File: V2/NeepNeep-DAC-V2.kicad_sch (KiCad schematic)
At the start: 18 parts, among them J1 Conn_02x03_Odd_Even, Q1 MMBT3904, U2 W25Q32JVSS, U3 ATtiny85-20SU

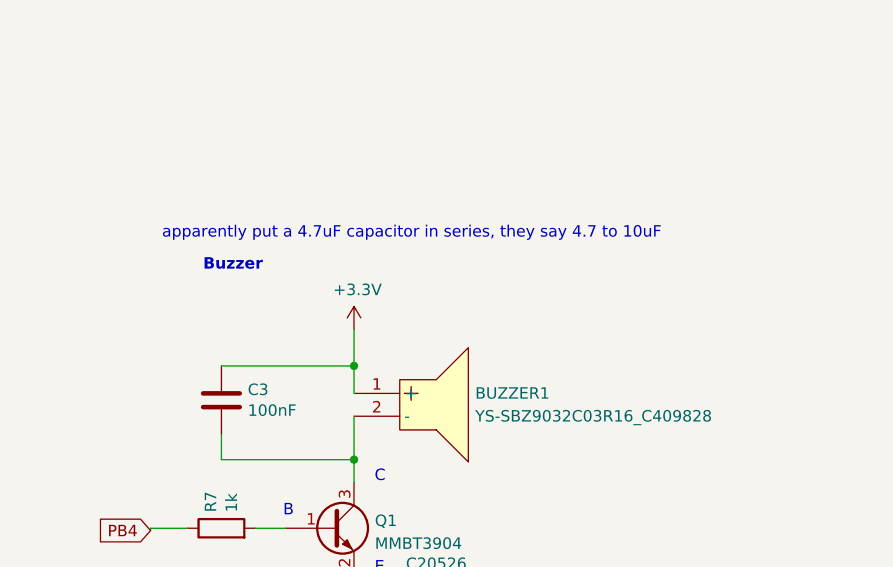
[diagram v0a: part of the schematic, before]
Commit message: Commit: M	NeepNeep-DAC-V1.kicad_sch A	V2/NeepNeep-DAC-V2-backups/NeepNeep-DAC-V2-2026-02-05_161125.zip A	V2/NeepNeep-DAC-V2-backups/NeepNeep-DAC-V2-2026-02-05_170153.zip A	V2/NeepNeep-DAC-V2.kicad_pcb A	V2/NeepNeep-DAC-V2.kicad_prl A	V2/NeepNeep-DAC-V2.kicad_pro A	V2/NeepNeep-DAC-V2.kicad_sch A	V2/fp-info-cache
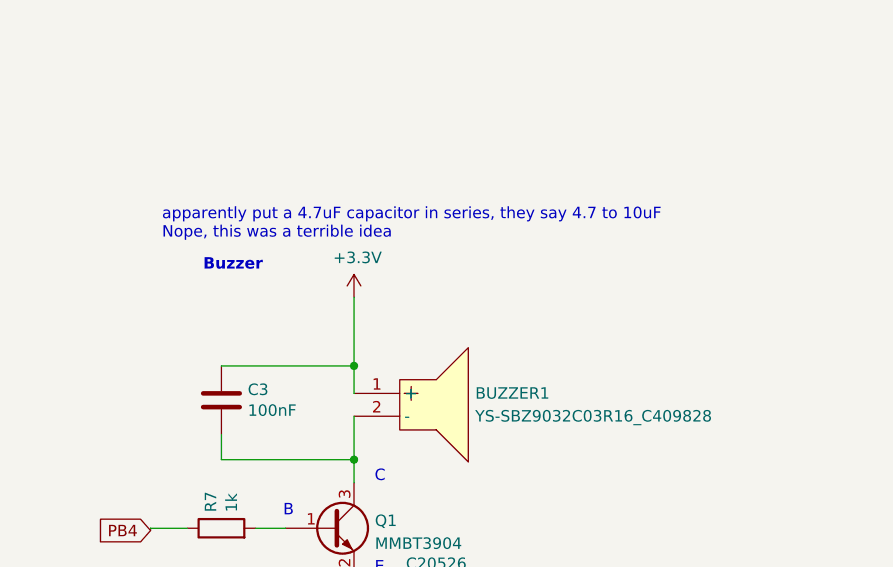
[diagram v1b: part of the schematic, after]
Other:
- note added: "apparently put a 4.7uF capacitor in series, they say 4.7 to 10uF Nope, this was a terrible idea"
- note removed: "apparently put a 4.7uF capacitor in series, they say 4.7 to 10uF"
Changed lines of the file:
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@@
   (junction (at 71.882 101.346) (diameter 0) (color 0 0 0 0)
   )
+  (junction (at 242.824 33.02) (diameter 0) (color 0 0 0 0)
+  )
   (junction (at 54.61 39.37) (diameter 0) (color 0 0 0 0)
   )
@@
   (junction (at 54.61 52.07) (diameter 0) (color 0 0 0 0)
   )
-  (junction (at 242.824 33.02) (diameter 0) (color 0 0 0 0)
-  )
   (junction (at 242.824 43.434) (diameter 0) (color 0 0 0 0)
   )
@@
     (stroke (width 0) (type default))
   )
+  (wire (pts (xy 242.824 25.4) (xy 242.824 33.02))
+    (stroke (width 0) (type default))
+  )
   (wire (pts (xy 60.325 52.07) (xy 54.61 52.07))
     (stroke (width 0) (type default))
@@
   )
   (wire (pts (xy 179.07 45.72) (xy 179.07 40.64))
-    (stroke (width 0) (type default))
-  )
-  (wire (pts (xy 242.824 28.956) (xy 242.824 33.02))
     (stroke (width 0) (type default))
   )
@@
     )
   )
-  (text "apparently put a 4.7uF capacitor in series, they say 4.7 to 10uF"
+  (text "apparently put a 4.7uF capacitor in series, they say 4.7 to 10uF\nNope, this was a terrible idea"
     (at 221.488 19.05 0)
     (effects (font (size 1.27 1.27)) (justify left bottom))
@@
     (pin "1")
     (instances
-      (project "NeepNeep-DAC-V1"
+      (project "NeepNeep-DAC-V2"
         (path "/53b8c8d9-463f-4715-b30d-544c8cc3c6e0"
           (reference "#PWR0101") (unit 1)
@@
     (pin "1")
     (instances
-      (project "NeepNeep-DAC-V1"
+      (project "NeepNeep-DAC-V2"
         (path "/53b8c8d9-463f-4715-b30d-544c8cc3c6e0"
           (reference "#PWR0102") (unit 1)
@@
     (pin "2")
     (instances
-      (project "NeepNeep-DAC-V1"
+      (project "NeepNeep-DAC-V2"
         (path "/53b8c8d9-463f-4715-b30d-544c8cc3c6e0"
           (reference "BT1") (unit 1)
@@
     (pin "1")
     (instances
-      (project "NeepNeep-DAC-V1"
+      (project "NeepNeep-DAC-V2"
         (path "/53b8c8d9-463f-4715-b30d-544c8cc3c6e0"
           (reference "#PWR0106") (unit 1)
@@
     (pin "1")
     (instances
-      (project "NeepNeep-DAC-V1"
+      (project "NeepNeep-DAC-V2"
         (path "/53b8c8d9-463f-4715-b30d-544c8cc3c6e0"
           (reference "#PWR0107") (unit 1)
@@
     (pin "2")
     (instances
-      (project "NeepNeep-DAC-V1"
+      (project "NeepNeep-DAC-V2"
         (path "/53b8c8d9-463f-4715-b30d-544c8cc3c6e0"
           (reference "C1") (unit 1)
@@
     (pin "1")
     (instances
-      (project "NeepNeep-DAC-V1"
+      (project "NeepNeep-DAC-V2"
         (path "/53b8c8d9-463f-4715-b30d-544c8cc3c6e0"
           (reference "#PWR0108") (unit 1)
@@
     (pin "2")
     (instances
-      (project "NeepNeep-DAC-V1"
+      (project "NeepNeep-DAC-V2"
         (path "/53b8c8d9-463f-4715-b30d-544c8cc3c6e0"
           (reference "C3") (unit 1)
@@
     (pin "2")
     (instances
-      (project "NeepNeep-DAC-V1"
+      (project "NeepNeep-DAC-V2"
         (path "/53b8c8d9-463f-4715-b30d-544c8cc3c6e0"
           (reference "R7") (unit 1)
@@
     (pin "1")
     (instances
-      (project "NeepNeep-DAC-V1"
+      (project "NeepNeep-DAC-V2"
         (path "/53b8c8d9-463f-4715-b30d-544c8cc3c6e0"
           (reference "#PWR0113") (unit 1)
@@
     (pin "1")
     (instances
-      (project "NeepNeep-DAC-V1"
+      (project "NeepNeep-DAC-V2"
         (path "/53b8c8d9-463f-4715-b30d-544c8cc3c6e0"
           (reference "#PWR0104") (unit 1)
@@
     (pin "3")
     (instances
-      (project "NeepNeep-DAC-V1"
+      (project "NeepNeep-DAC-V2"
         (path "/53b8c8d9-463f-4715-b30d-544c8cc3c6e0"
           (reference "U2") (unit 1)
@@
     (pin "3")
     (instances
-      (project "NeepNeep-DAC-V1"
+      (project "NeepNeep-DAC-V2"
         (path "/53b8c8d9-463f-4715-b30d-544c8cc3c6e0"
           (reference "Q1") (unit 1)
@@
     (pin "1")
     (instances
-      (project "NeepNeep-DAC-V1"
+      (project "NeepNeep-DAC-V2"
         (path "/53b8c8d9-463f-4715-b30d-544c8cc3c6e0"
           (reference "#PWR02") (unit 1)
@@
     (pin "2")
     (instances
-      (project "NeepNeep-DAC-V1"
+      (project "NeepNeep-DAC-V2"
         (path "/53b8c8d9-463f-4715-b30d-544c8cc3c6e0"
           (reference "R2") (unit 1)
@@
     (pin "2")
     (instances
-      (project "NeepNeep-DAC-V1"
+      (project "NeepNeep-DAC-V2"
         (path "/53b8c8d9-463f-4715-b30d-544c8cc3c6e0"
           (reference "D1") (unit 1)
@@
     (pin "7")
     (instances
-      (project "NeepNeep-DAC-V1"
+      (project "NeepNeep-DAC-V2"
         (path "/53b8c8d9-463f-4715-b30d-544c8cc3c6e0"
           (reference "U3") (unit 1)
@@
     (pin "6")
     (instances
-      (project "NeepNeep-DAC-V1"
+      (project "NeepNeep-DAC-V2"
         (path "/53b8c8d9-463f-4715-b30d-544c8cc3c6e0"
           (reference "J1") (unit 1)
@@
     (pin "1")
     (instances
-      (project "NeepNeep-DAC-V1"
+      (project "NeepNeep-DAC-V2"
         (path "/53b8c8d9-463f-4715-b30d-544c8cc3c6e0"
           (reference "#PWR0115") (unit 1)
@@
     (pin "1")
     (instances
-      (project "NeepNeep-DAC-V1"
+      (project "NeepNeep-DAC-V2"
         (path "/53b8c8d9-463f-4715-b30d-544c8cc3c6e0"
           (reference "#PWR0110") (unit 1)
@@
     (pin "2")
     (instances
-      (project "NeepNeep-DAC-V1"
+      (project "NeepNeep-DAC-V2"
         (path "/53b8c8d9-463f-4715-b30d-544c8cc3c6e0"
           (reference "R1") (unit 1)
@@
     (pin "2")
     (instances
-      (project "NeepNeep-DAC-V1"
+      (project "NeepNeep-DAC-V2"
         (path "/53b8c8d9-463f-4715-b30d-544c8cc3c6e0"
           (reference "D3") (unit 1)
@@
     )
   )
-  (symbol (lib_id "power:+3.3V") (at 242.824 28.956 0) (unit 1)
-    (in_bom yes) (on_board yes) (dnp no)
-    (property "Reference" "#PWR0114" (at 242.824 32.766 0)
-      (effects (font (size 1.27 1.27)) hide)
-    )
-    (property "Value" "+3.3V" (at 243.205 24.5618 0)
-      (effects (font (size 1.27 1.27)))
-    )
-    (property "Footprint" "" (at 242.824 28.956 0)
-      (effects (font (size 1.27 1.27)) hide)
-    )
-    (property "Datasheet" "" (at 242.824 28.956 0)
-      (effects (font (size 1.27 1.27)) hide)
-    )
-    (pin "1")
-    (instances
-      (project "NeepNeep-DAC-V1"
+  (symbol (lib_id "power:+3.3V") (at 242.824 25.4 0) (unit 1)
+    (in_bom yes) (on_board yes) (dnp no)
+    (property "Reference" "#PWR0114" (at 242.824 29.21 0)
+      (effects (font (size 1.27 1.27)) hide)
+    )
+    (property "Value" "+3.3V" (at 243.205 21.0058 0)
+      (effects (font (size 1.27 1.27)))
+    )
+    (property "Footprint" "" (at 242.824 25.4 0)
+      (effects (font (size 1.27 1.27)) hide)
+    )
+    (property "Datasheet" "" (at 242.824 25.4 0)
+      (effects (font (size 1.27 1.27)) hide)
+    )
+    (pin "1")
+    (instances
+      (project "NeepNeep-DAC-V2"
         (path "/53b8c8d9-463f-4715-b30d-544c8cc3c6e0"
           (reference "#PWR0114") (unit 1)
@@
     (pin "2")
     (instances
-      (project "NeepNeep-DAC-V1"
+      (project "NeepNeep-DAC-V2"
         (path "/53b8c8d9-463f-4715-b30d-544c8cc3c6e0"
           (reference "D2") (unit 1)
@@
     (pin "1")
     (instances
-      (project "NeepNeep-DAC-V1"
+      (project "NeepNeep-DAC-V2"
         (path "/53b8c8d9-463f-4715-b30d-544c8cc3c6e0"
           (reference "#PWR05") (unit 1)
@@
     (pin "2")
     (instances
-      (project "NeepNeep-DAC-V1"
+      (project "NeepNeep-DAC-V2"
         (path "/53b8c8d9-463f-4715-b30d-544c8cc3c6e0"
           (reference "R6") (unit 1)
@@
     (pin "2")
     (instances
-      (project "NeepNeep-DAC-V1"
+      (project "NeepNeep-DAC-V2"
         (path "/53b8c8d9-463f-4715-b30d-544c8cc3c6e0"
           (reference "C4") (unit 1)
@@
     (pin "2")
     (instances
-      (project "NeepNeep-DAC-V1"
+      (project "NeepNeep-DAC-V2"
         (path "/53b8c8d9-463f-4715-b30d-544c8cc3c6e0"
           (reference "C2") (unit 1)
@@
     (pin "1")
     (instances
-      (project "NeepNeep-DAC-V1"
+      (project "NeepNeep-DAC-V2"
         (path "/53b8c8d9-463f-4715-b30d-544c8cc3c6e0"
           (reference "#PWR03") (unit 1)
@@
     (pin "2")
     (instances
-      (project "NeepNeep-DAC-V1"
+      (project "NeepNeep-DAC-V2"
         (path "/53b8c8d9-463f-4715-b30d-544c8cc3c6e0"
           (reference "R3") (unit 1)
@@
     (pin "1")
     (instances
-      (project "NeepNeep-DAC-V1"
+      (project "NeepNeep-DAC-V2"
         (path "/53b8c8d9-463f-4715-b30d-544c8cc3c6e0"
           (reference "#PWR0112") (unit 1)
@@
     (pin "1")
     (instances
-      (project "NeepNeep-DAC-V1"
+      (project "NeepNeep-DAC-V2"
         (path "/53b8c8d9-463f-4715-b30d-544c8cc3c6e0"
           (reference "BUZZER1") (unit 1)
@@
     (pin "1")
     (instances
-      (project "NeepNeep-DAC-V1"
+      (project "NeepNeep-DAC-V2"
         (path "/53b8c8d9-463f-4715-b30d-544c8cc3c6e0"
           (reference "#PWR01") (unit 1)
@@
     (pin "1")
     (instances
-      (project "NeepNeep-DAC-V1"
+      (project "NeepNeep-DAC-V2"
         (path "/53b8c8d9-463f-4715-b30d-544c8cc3c6e0"
           (reference "#PWR04") (unit 1)
